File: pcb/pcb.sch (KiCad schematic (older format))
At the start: 141 parts, among them SW1 SW_Push, U1 PRTR5V0U2X, U2 ATmega32U4-AU, Y1 16MHz

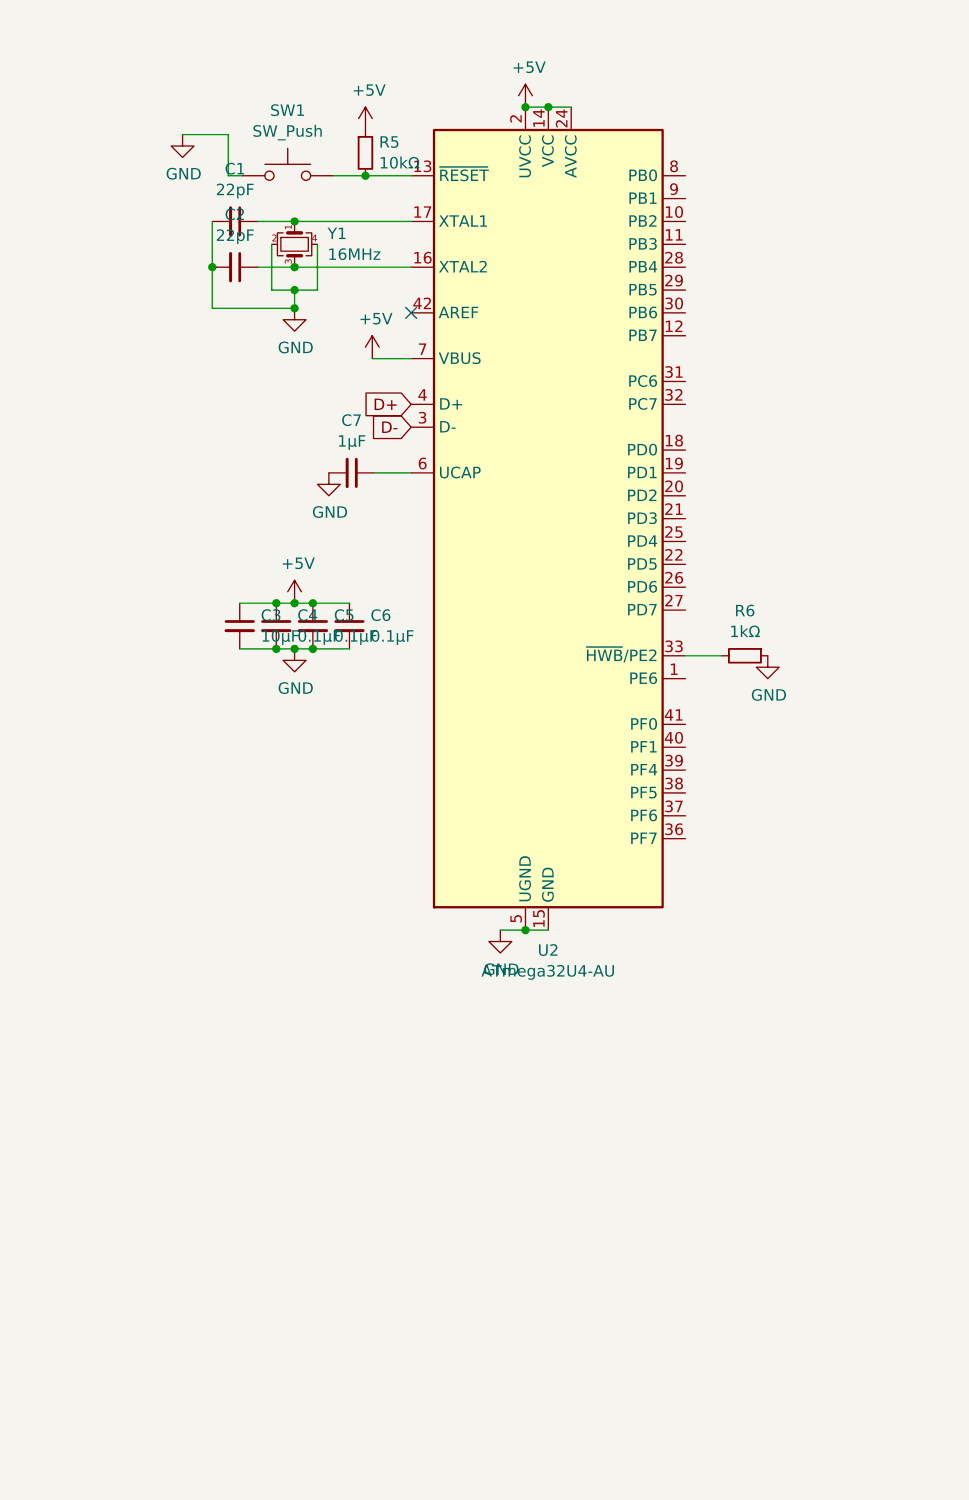
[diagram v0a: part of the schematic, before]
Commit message: finished rev 1 PCB
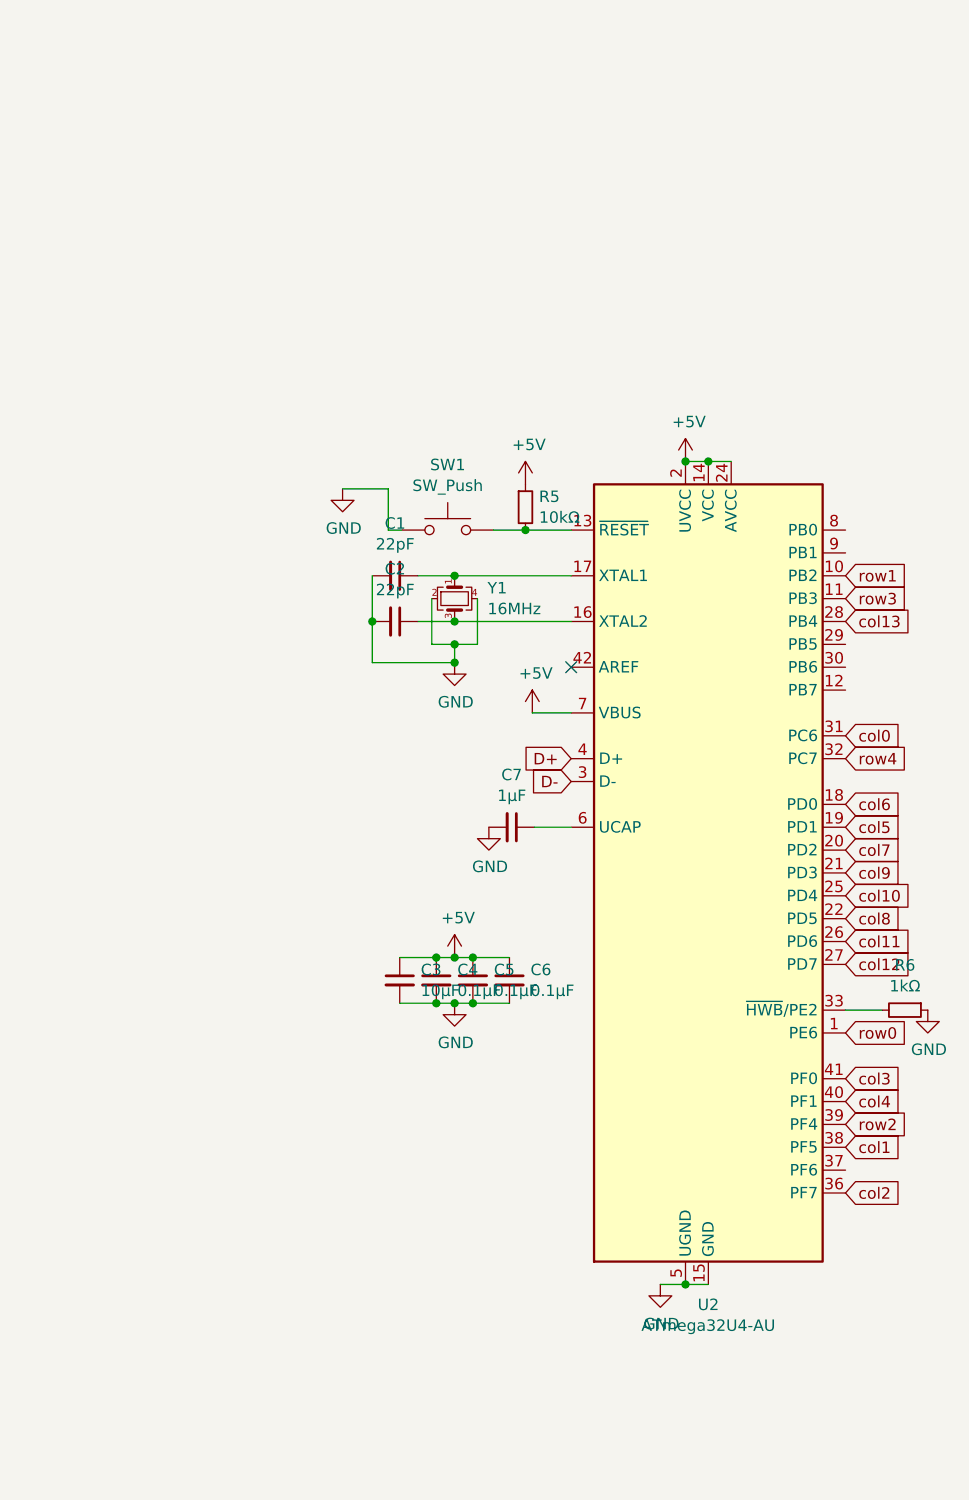
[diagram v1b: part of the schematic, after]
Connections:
- net col0: now also U2.31 (PC6)
- net col1: now also U2.38 (PF5)
- net col10: now also U2.25 (PD4)
- net col11: now also U2.26 (PD6)
- net col12: now also U2.27 (PD7)
- net col13: now also U2.28 (PB4)
- net col2: now also U2.36 (PF7)
- net col3: now also U2.41 (PF0)
- net col4: now also U2.40 (PF1)
- net col5: now also U2.19 (PD1)
- net col6: now also U2.18 (PD0)
- net col7: now also U2.20 (PD2)
- net col8: now also U2.22 (PD5)
- net col9: now also U2.21 (PD3)
- net row0: now also U2.1 (PE6)
- net row1: now also U2.10 (PB2)
- net row2: now also U2.39 (PF4)
- net row3: now also U2.11 (PB3)
- net row4: now also U2.32 (PC7)
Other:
- moved on the sheet: C1, C2, C3, C4, C5, C6, C7, R5, R6, SW1, U2, Y1

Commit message: whatever update was done
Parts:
- MX1, MX10, MX11, MX12, MX13, MX14, MX15, MX16, MX17, MX18, MX19, MX2, MX20, MX21, MX22, MX23, MX24, MX25, MX26, MX27, MX28, MX29, MX3, MX30, MX31, MX32, MX33, MX34, MX35, MX36, MX37, MX38, MX39, MX4, MX40, MX41, MX42, MX43, MX44, MX45, MX46, MX47, MX48, MX49, MX5, MX50, MX51, MX52, MX53, MX54, MX55, MX56, MX57, MX58, MX59, MX6, MX60, MX61, MX7, MX8, MX9: symbol MX_Alps_Hybrid:MX-NoLED -> pcb-rescue:MX-NoLED-MX_Alps_Hybrid
- U1: symbol random-keyboard-parts:PRTR5V0U2X -> pcb-rescue:PRTR5V0U2X-random-keyboard-parts
- USB1: symbol keebio:HRO-TYPE-C-31-M-12 -> pcb-rescue:HRO-TYPE-C-31-M-12-keebio
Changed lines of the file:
@@
 Connection ~ 9920 2390
 $Comp
-L keebio:HRO-TYPE-C-31-M-12 USB1
+L pcb-rescue:HRO-TYPE-C-31-M-12-keebio USB1
 U 1 1 60B21C59
 P 2230 6040
@@
 $EndComp
 $Comp
-L random-keyboard-parts:PRTR5V0U2X U1
+L pcb-rescue:PRTR5V0U2X-random-keyboard-parts U1
 U 1 1 60B226B5
 P 3710 6270
@@
 D-
 $Comp
-L MX_Alps_Hybrid:MX-NoLED MX1
+L pcb-rescue:MX-NoLED-MX_Alps_Hybrid MX1
 U 1 1 60B503F2
 P 790 870
@@
 $EndComp
 $Comp
-L MX_Alps_Hybrid:MX-NoLED MX6
+L pcb-rescue:MX-NoLED-MX_Alps_Hybrid MX6
 U 1 1 60B59A7A
 P 1090 870
@@
 $EndComp
 $Comp
-L MX_Alps_Hybrid:MX-NoLED MX10
+L pcb-rescue:MX-NoLED-MX_Alps_Hybrid MX10
 U 1 1 60B5C36E
 P 1390 870
@@
 $EndComp
 $Comp
-L MX_Alps_Hybrid:MX-NoLED MX15
+L pcb-rescue:MX-NoLED-MX_Alps_Hybrid MX15
 U 1 1 60B5EF8C
 P 1690 870
@@
 $EndComp
 $Comp
-L MX_Alps_Hybrid:MX-NoLED MX19
+L pcb-rescue:MX-NoLED-MX_Alps_Hybrid MX19
 U 1 1 60B61B17
 P 1990 870
@@
 $EndComp
 $Comp
-L MX_Alps_Hybrid:MX-NoLED MX23
+L pcb-rescue:MX-NoLED-MX_Alps_Hybrid MX23
 U 1 1 60B6486A
 P 2290 870
@@
 $EndComp
 $Comp
-L MX_Alps_Hybrid:MX-NoLED MX27
+L pcb-rescue:MX-NoLED-MX_Alps_Hybrid MX27
 U 1 1 60B67A58
 P 2590 870
@@
 $EndComp
 $Comp
-L MX_Alps_Hybrid:MX-NoLED MX32
+L pcb-rescue:MX-NoLED-MX_Alps_Hybrid MX32
 U 1 1 60B6A9C0
 P 2890 870
@@
 $EndComp
 $Comp
-L MX_Alps_Hybrid:MX-NoLED MX36
+L pcb-rescue:MX-NoLED-MX_Alps_Hybrid MX36
 U 1 1 60B6DA5C
 P 3190 870
@@
 $EndComp
 $Comp
-L MX_Alps_Hybrid:MX-NoLED MX40
+L pcb-rescue:MX-NoLED-MX_Alps_Hybrid MX40
 U 1 1 60B70C9E
 P 3490 870
@@
 $EndComp
 $Comp
-L MX_Alps_Hybrid:MX-NoLED MX44
+L pcb-rescue:MX-NoLED-MX_Alps_Hybrid MX44
 U 1 1 60B73F84
 P 3790 870
@@
 $EndComp
 $Comp
-L MX_Alps_Hybrid:MX-NoLED MX49
+L pcb-rescue:MX-NoLED-MX_Alps_Hybrid MX49
 U 1 1 60B7A762
 P 4090 870
@@
 $EndComp
 $Comp
-L MX_Alps_Hybrid:MX-NoLED MX54
+L pcb-rescue:MX-NoLED-MX_Alps_Hybrid MX54
 U 1 1 60B7DC89
 P 4390 870
@@
 $EndComp
 $Comp
-L MX_Alps_Hybrid:MX-NoLED MX57
+L pcb-rescue:MX-NoLED-MX_Alps_Hybrid MX57
 U 1 1 60B81433
 P 4690 870
@@
 $EndComp
 $Comp
-L MX_Alps_Hybrid:MX-NoLED MX2
+L pcb-rescue:MX-NoLED-MX_Alps_Hybrid MX2
 U 1 1 60B999F5
 P 790 1470
@@
 	740  1620 690  1620
 $Comp
-L MX_Alps_Hybrid:MX-NoLED MX7
+L pcb-rescue:MX-NoLED-MX_Alps_Hybrid MX7
 U 1 1 60B99A02
 P 1090 1470
@@
 $EndComp
 $Comp
-L MX_Alps_Hybrid:MX-NoLED MX11
+L pcb-rescue:MX-NoLED-MX_Alps_Hybrid MX11
 U 1 1 60B99A0F
 P 1390 1470
@@
 $EndComp
 $Comp
-L MX_Alps_Hybrid:MX-NoLED MX16
+L pcb-rescue:MX-NoLED-MX_Alps_Hybrid MX16
 U 1 1 60B99A1C
 P 1690 1470
@@
 $EndComp
 $Comp
-L MX_Alps_Hybrid:MX-NoLED MX20
+L pcb-rescue:MX-NoLED-MX_Alps_Hybrid MX20
 U 1 1 60B99A29
 P 1990 1470
@@
 $EndComp
 $Comp
-L MX_Alps_Hybrid:MX-NoLED MX24
+L pcb-rescue:MX-NoLED-MX_Alps_Hybrid MX24
 U 1 1 60B99A36
 P 2290 1470
@@
 $EndComp
 $Comp
-L MX_Alps_Hybrid:MX-NoLED MX28
+L pcb-rescue:MX-NoLED-MX_Alps_Hybrid MX28
 U 1 1 60B99A43
 P 2590 1470
@@
 $EndComp
 $Comp
-L MX_Alps_Hybrid:MX-NoLED MX33
+L pcb-rescue:MX-NoLED-MX_Alps_Hybrid MX33
 U 1 1 60B99A50
 P 2890 1470
@@
 $EndComp
 $Comp
-L MX_Alps_Hybrid:MX-NoLED MX37
+L pcb-rescue:MX-NoLED-MX_Alps_Hybrid MX37
 U 1 1 60B99A5D
 P 3190 1470
@@
 $EndComp
 $Comp
-L MX_Alps_Hybrid:MX-NoLED MX41
+L pcb-rescue:MX-NoLED-MX_Alps_Hybrid MX41
 U 1 1 60B99A6A
 P 3490 1470
@@
 $EndComp
 $Comp
-L MX_Alps_Hybrid:MX-NoLED MX45
+L pcb-rescue:MX-NoLED-MX_Alps_Hybrid MX45
 U 1 1 60B99A77
 P 3790 1470
@@
 $EndComp
 $Comp
-L MX_Alps_Hybrid:MX-NoLED MX50
+L pcb-rescue:MX-NoLED-MX_Alps_Hybrid MX50
 U 1 1 60B99A84
 P 4090 1470
@@
 $EndComp
 $Comp
-L MX_Alps_Hybrid:MX-NoLED MX55
+L pcb-rescue:MX-NoLED-MX_Alps_Hybrid MX55
 U 1 1 60B99A91
 P 4390 1470
@@
 $EndComp
 $Comp
-L MX_Alps_Hybrid:MX-NoLED MX58
+L pcb-rescue:MX-NoLED-MX_Alps_Hybrid MX58
 U 1 1 60B99A9E
 P 4690 1470
@@
 $EndComp
 $Comp
-L MX_Alps_Hybrid:MX-NoLED MX3
+L pcb-rescue:MX-NoLED-MX_Alps_Hybrid MX3
 U 1 1 60BAA3AF
 P 790 2070
@@
 $EndComp
 $Comp
-L MX_Alps_Hybrid:MX-NoLED MX8
+L pcb-rescue:MX-NoLED-MX_Alps_Hybrid MX8
 U 1 1 60BAA3BC
 P 1090 2070
@@
 $EndComp
 $Comp
-L MX_Alps_Hybrid:MX-NoLED MX12
+L pcb-rescue:MX-NoLED-MX_Alps_Hybrid MX12
 U 1 1 60BAA3C9
 P 1390 2070
@@
 $EndComp
 $Comp
-L MX_Alps_Hybrid:MX-NoLED MX17
+L pcb-rescue:MX-NoLED-MX_Alps_Hybrid MX17
 U 1 1 60BAA3D6
 P 1690 2070
@@
 $EndComp
 $Comp
-L MX_Alps_Hybrid:MX-NoLED MX21
+L pcb-rescue:MX-NoLED-MX_Alps_Hybrid MX21
 U 1 1 60BAA3E3
 P 1990 2070
@@
 $EndComp
 $Comp
-L MX_Alps_Hybrid:MX-NoLED MX25
+L pcb-rescue:MX-NoLED-MX_Alps_Hybrid MX25
 U 1 1 60BAA3F0
 P 2290 2070
@@
 $EndComp
 $Comp
-L MX_Alps_Hybrid:MX-NoLED MX29
+L pcb-rescue:MX-NoLED-MX_Alps_Hybrid MX29
 U 1 1 60BAA3FD
 P 2590 2070
@@
 $EndComp
 $Comp
-L MX_Alps_Hybrid:MX-NoLED MX34
+L pcb-rescue:MX-NoLED-MX_Alps_Hybrid MX34
 U 1 1 60BAA40A
 P 2890 2070
@@
 $EndComp
 $Comp
-L MX_Alps_Hybrid:MX-NoLED MX38
+L pcb-rescue:MX-NoLED-MX_Alps_Hybrid MX38
 U 1 1 60BAA417
 P 3190 2070
@@
 $EndComp
 $Comp
-L MX_Alps_Hybrid:MX-NoLED MX42
+L pcb-rescue:MX-NoLED-MX_Alps_Hybrid MX42
 U 1 1 60BAA424
 P 3490 2070
@@
 $EndComp
 $Comp
-L MX_Alps_Hybrid:MX-NoLED MX46
+L pcb-rescue:MX-NoLED-MX_Alps_Hybrid MX46
 U 1 1 60BAA431
 P 3790 2070
@@
 $EndComp
 $Comp
-L MX_Alps_Hybrid:MX-NoLED MX51
+L pcb-rescue:MX-NoLED-MX_Alps_Hybrid MX51
 U 1 1 60BAA43E
 P 4090 2070
@@
 $EndComp
 $Comp
-L MX_Alps_Hybrid:MX-NoLED MX59
+L pcb-rescue:MX-NoLED-MX_Alps_Hybrid MX59
 U 1 1 60BAA44B
 P 4690 2070
@@
 $EndComp
 $Comp
-L MX_Alps_Hybrid:MX-NoLED MX4
+L pcb-rescue:MX-NoLED-MX_Alps_Hybrid MX4
 U 1 1 60BBE0C3
 P 790 2670
@@
 $EndComp
 $Comp
-L MX_Alps_Hybrid:MX-NoLED MX60
+L pcb-rescue:MX-NoLED-MX_Alps_Hybrid MX60
 U 1 1 60BBE152
 P 4690 2670
@@
 $EndComp
 $Comp
-L MX_Alps_Hybrid:MX-NoLED MX5
+L pcb-rescue:MX-NoLED-MX_Alps_Hybrid MX5
 U 1 1 60BD5BDC
 P 790 3270
@@
 $EndComp
 $Comp
-L MX_Alps_Hybrid:MX-NoLED MX9
+L pcb-rescue:MX-NoLED-MX_Alps_Hybrid MX9
 U 1 1 60BD5BE9
 P 1090 3270
@@
 $EndComp
 $Comp
-L MX_Alps_Hybrid:MX-NoLED MX14
+L pcb-rescue:MX-NoLED-MX_Alps_Hybrid MX14
 U 1 1 60BD5BF6
 P 1390 3270
@@
 $EndComp
 $Comp
-L MX_Alps_Hybrid:MX-NoLED MX31
+L pcb-rescue:MX-NoLED-MX_Alps_Hybrid MX31
 U 1 1 60BD5C03
 P 2590 3270
@@
 $EndComp
 $Comp
-L MX_Alps_Hybrid:MX-NoLED MX48
+L pcb-rescue:MX-NoLED-MX_Alps_Hybrid MX48
 U 1 1 60BD5C10
 P 3790 3270
@@
 $EndComp
 $Comp
-L MX_Alps_Hybrid:MX-NoLED MX53
+L pcb-rescue:MX-NoLED-MX_Alps_Hybrid MX53
 U 1 1 60BD5C1D
 P 4090 3270
@@
 $EndComp
 $Comp
-L MX_Alps_Hybrid:MX-NoLED MX56
+L pcb-rescue:MX-NoLED-MX_Alps_Hybrid MX56
 U 1 1 60BD5C2A
 P 4390 3270
@@
 $EndComp
 $Comp
-L MX_Alps_Hybrid:MX-NoLED MX61
+L pcb-rescue:MX-NoLED-MX_Alps_Hybrid MX61
 U 1 1 60BD5C37
 P 4690 3270
@@
 	4040 2820 3990 2820
 $Comp
-L MX_Alps_Hybrid:MX-NoLED MX52
+L pcb-rescue:MX-NoLED-MX_Alps_Hybrid MX52
 U 1 1 60BBE145
 P 4090 2670
@@
 	3740 2820 3690 2820
 $Comp
-L MX_Alps_Hybrid:MX-NoLED MX47
+L pcb-rescue:MX-NoLED-MX_Alps_Hybrid MX47
 U 1 1 60BBE138
 P 3790 2670
@@
 	3440 2820 3390 2820
 $Comp
-L MX_Alps_Hybrid:MX-NoLED MX43
+L pcb-rescue:MX-NoLED-MX_Alps_Hybrid MX43
 U 1 1 60BBE12B
 P 3490 2670
@@
 	3140 2820 3090 2820
 $Comp
-L MX_Alps_Hybrid:MX-NoLED MX39
+L pcb-rescue:MX-NoLED-MX_Alps_Hybrid MX39
 U 1 1 60BBE11E
 P 3190 2670
@@
 	2840 2820 2790 2820
 $Comp
-L MX_Alps_Hybrid:MX-NoLED MX35
+L pcb-rescue:MX-NoLED-MX_Alps_Hybrid MX35
 U 1 1 60BBE111
 P 2890 2670
@@
 	2540 2820 2490 2820
 $Comp
-L MX_Alps_Hybrid:MX-NoLED MX30
+L pcb-rescue:MX-NoLED-MX_Alps_Hybrid MX30
 U 1 1 60BBE104
 P 2590 2670
@@
 	2240 2820 2190 2820
 $Comp
-L MX_Alps_Hybrid:MX-NoLED MX26
+L pcb-rescue:MX-NoLED-MX_Alps_Hybrid MX26
 U 1 1 60BBE0F7
 P 2290 2670
@@
 	1940 2820 1890 2820
 $Comp
-L MX_Alps_Hybrid:MX-NoLED MX22
+L pcb-rescue:MX-NoLED-MX_Alps_Hybrid MX22
 U 1 1 60BBE0EA
 P 1990 2670
@@
 	1640 2820 1590 2820
 $Comp
-L MX_Alps_Hybrid:MX-NoLED MX18
+L pcb-rescue:MX-NoLED-MX_Alps_Hybrid MX18
 U 1 1 60BBE0DD
 P 1690 2670
@@
 	1340 2820 1290 2820
 $Comp
-L MX_Alps_Hybrid:MX-NoLED MX13
+L pcb-rescue:MX-NoLED-MX_Alps_Hybrid MX13
 U 1 1 60BBE0D0
 P 1390 2670
